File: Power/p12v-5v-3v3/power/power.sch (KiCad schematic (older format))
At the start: 19 parts, among them U1 ASM1117-3V3, U2 MP1584

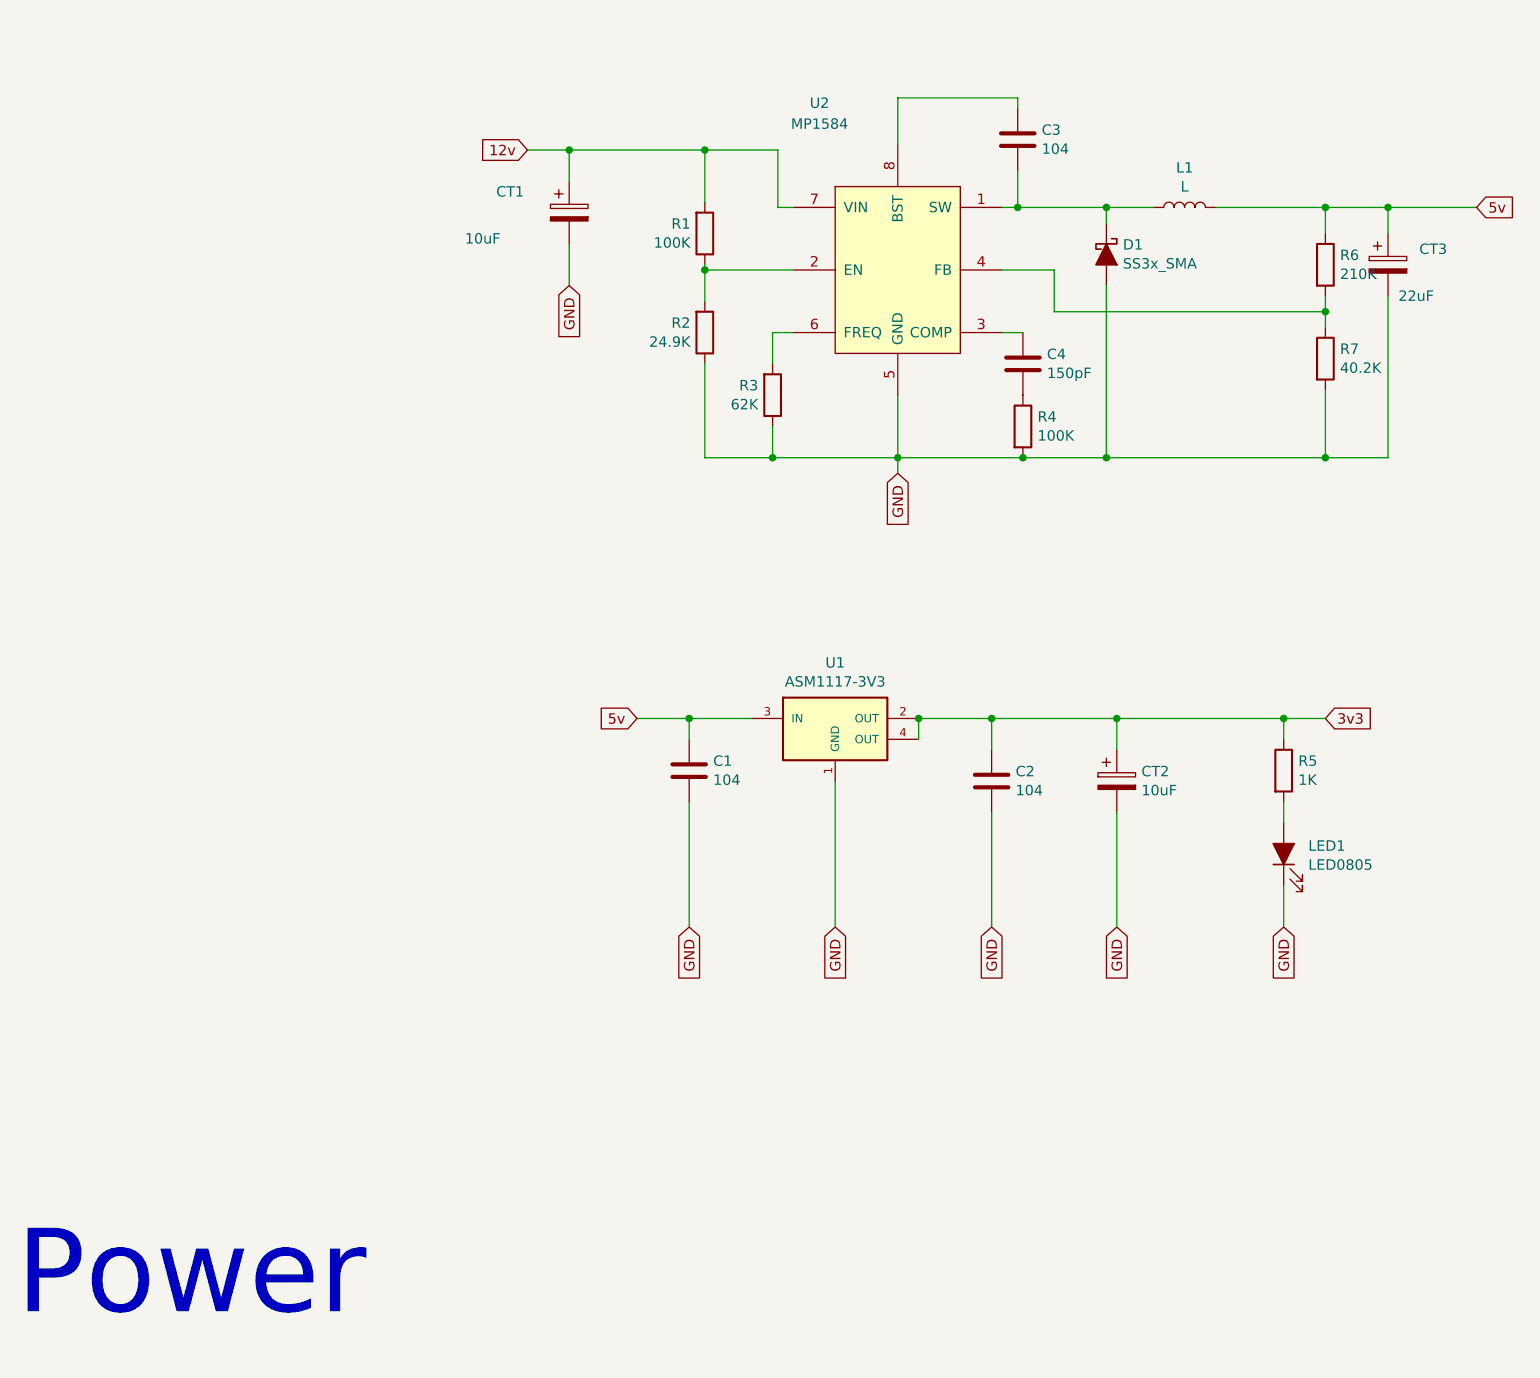
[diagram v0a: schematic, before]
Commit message: add
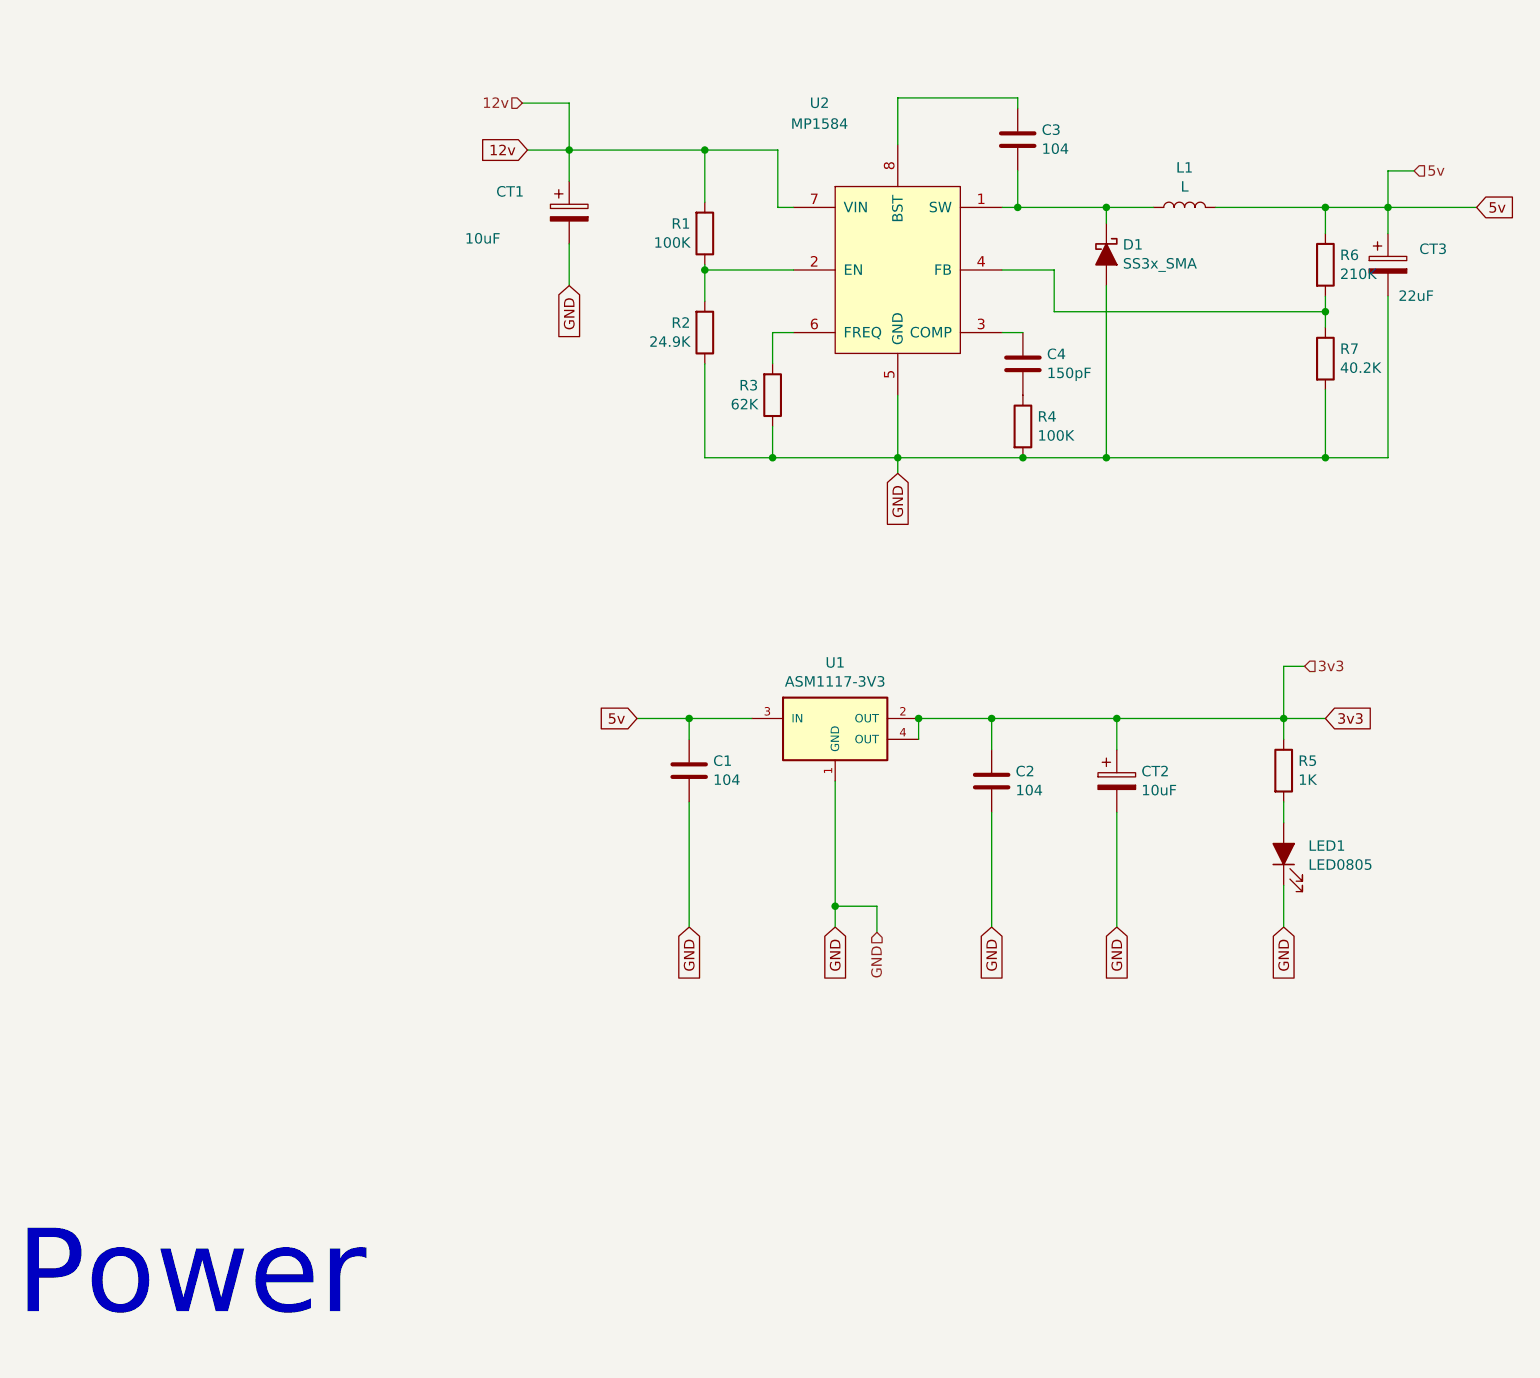
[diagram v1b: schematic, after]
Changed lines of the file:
@@
 EESchema Schematic File Version 4
-LIBS:ph_do_controller_hw-cache
-LIBS:ph_stm32_single_parameter_lcd_132x64_hw-cache
+LIBS:power-cache
 EELAYER 30 0
 EELAYER END
@@
 	4075 4900 4075 5500
 Wire Wire Line
-	4775 4800 4775 5500
+	4775 4800 4775 5400
 Wire Wire Line
 	5525 4950 5525 5500
@@
 	0    -1   -1   0
 $EndComp
+Text HLabel 7025 4250 2    50   Input ~ 0
+3v3
+Wire Wire Line
+	7025 4250 6925 4250
+Wire Wire Line
+	6925 4250 6925 4500
+Text HLabel 7550 1875 2    50   Input ~ 0
+5v
+Wire Wire Line
+	7550 1875 7425 1875
+Wire Wire Line
+	7425 1875 7425 2050
+Text HLabel 3275 1550 0    50   Input ~ 0
+12v
+Wire Wire Line
+	3275 1550 3500 1550
+Wire Wire Line
+	3500 1550 3500 1775
+Text HLabel 4975 5525 3    50   Input ~ 0
+GND
+Wire Wire Line
+	4975 5525 4975 5400
+Wire Wire Line
+	4975 5400 4775 5400
+Connection ~ 4775 5400
+Wire Wire Line
+	4775 5400 4775 5500
 $EndSCHEMATC

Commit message: update
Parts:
- removed C1, C2, C3: 104, ph_kicad_lib:C_0805_HandSoldering, symbol ph_kicad_lib:C0805
- removed C4: 150pF, ph_kicad_lib:C_0805_HandSoldering, symbol ph_kicad_lib:C0805
- removed CT1, CT2: 10uF, ph_kicad_lib:CP_Tantalum_Case-B_EIA-3528-21_Reflow, symbol ph_kicad_lib:CT_3528
- removed CT3: 22uF, ph_kicad_lib:CP_Tantalum_Case-B_EIA-3528-21_Reflow, symbol ph_kicad_lib:CT_3528
- removed D1: SS3x_SMA, ph_kicad_lib:D_SMA, symbol ph_kicad_lib:SS3x_SMA
- removed L1: L, ph_kicad_lib:L_5D28_HandSoldering, symbol Device:L
- removed LED1: LED0805, ph_kicad_lib:LED_0805, symbol ph_kicad_lib:LED0805
- removed R1, R4: 100K, ph_kicad_lib:R_0805_HandSoldering, symbol ph_kicad_lib:R0805
- removed R2: 24.9K, ph_kicad_lib:R_0805_HandSoldering, symbol ph_kicad_lib:R0805
- removed R3: 62K, ph_kicad_lib:R_0805_HandSoldering, symbol ph_kicad_lib:R0805
- removed R5: 1K, ph_kicad_lib:R_0805_HandSoldering, symbol ph_kicad_lib:R0805
- removed R6: 210K, ph_kicad_lib:R_0805_HandSoldering, symbol ph_kicad_lib:R0805
- removed R7: 40.2K, ph_kicad_lib:R_0603_HandSoldering, symbol ph_kicad_lib:R0603
- removed U2: MP1584, ph_kicad_lib:SOIC-8-1EP_3.9x4.9mm_Pitch1.27mm, symbol ph_kicad_lib:MP1584
- added C1, C2, C3: 104, phuong_kicad_lib:C_0805, symbol phuong-kicad-lib:C0805
- added C4: 150p, phuong_kicad_lib:C_0805, symbol phuong-kicad-lib:C0805
- added CP1, CP2: 10uF, phuong_kicad_lib:CP_Tatanlum_1206_3216, symbol phuong-kicad-lib:C-Tantalum-1206
- added CP3: 20uF, phuong_kicad_lib:CP_Tatanlum_1206_3216, symbol phuong-kicad-lib:C-Tantalum-1206
- added D1: SS3x_SMA, phuong_kicad_lib:D_SMA, symbol phuong-kicad-lib:SS3x_SMA
- added L1: L_5D28, phuong_kicad_lib:L_5D28_HandSoldering, symbol phuong-kicad-lib:L_5D28
- added Led1: Led_0805, phuong_kicad_lib:LED_0805, symbol phuong-kicad-lib:Led_0805
- added R1, R4: 100k, phuong_kicad_lib:R_0805, symbol phuong-kicad-lib:R0805
- added R2: 24.9k, phuong_kicad_lib:R_0805, symbol phuong-kicad-lib:R0805
- added R3: 62k, phuong_kicad_lib:R_0805, symbol phuong-kicad-lib:R0805
- added R5: 1k, phuong_kicad_lib:R_0805, symbol phuong-kicad-lib:R0805
- added R6: 210k, phuong_kicad_lib:R_0805, symbol phuong-kicad-lib:R0805
- added R7: 40.2k, phuong_kicad_lib:R_0805, symbol phuong-kicad-lib:R0805
- added U2: MP1584, phuong_kicad_lib:SOIC-8_3.9x4.9mm_Pitch1.27mm, symbol phuong-kicad-lib:MP1584
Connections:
- wire segments 71 -> 70
